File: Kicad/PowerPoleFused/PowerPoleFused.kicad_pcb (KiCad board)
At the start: 2 copper layers, 96.5 x 43.2 mm, 12 parts, among them J1 Anderson powerpole, J2 Anderson powerpole, J3 Anderson powerpole, J4 Anderson powerpole, J5 Anderson powerpole, J6 Anderson powerpole

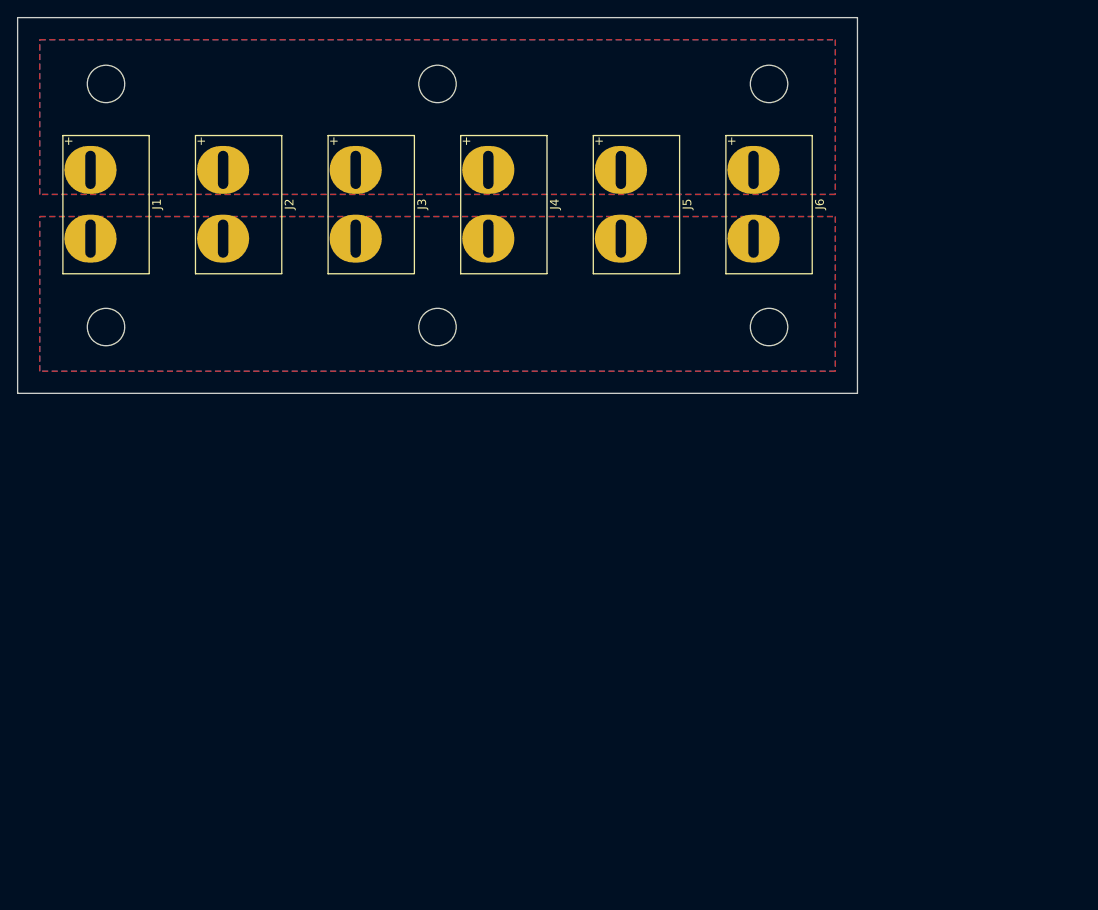
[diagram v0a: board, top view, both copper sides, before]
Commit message: Laid out board 1st attempt
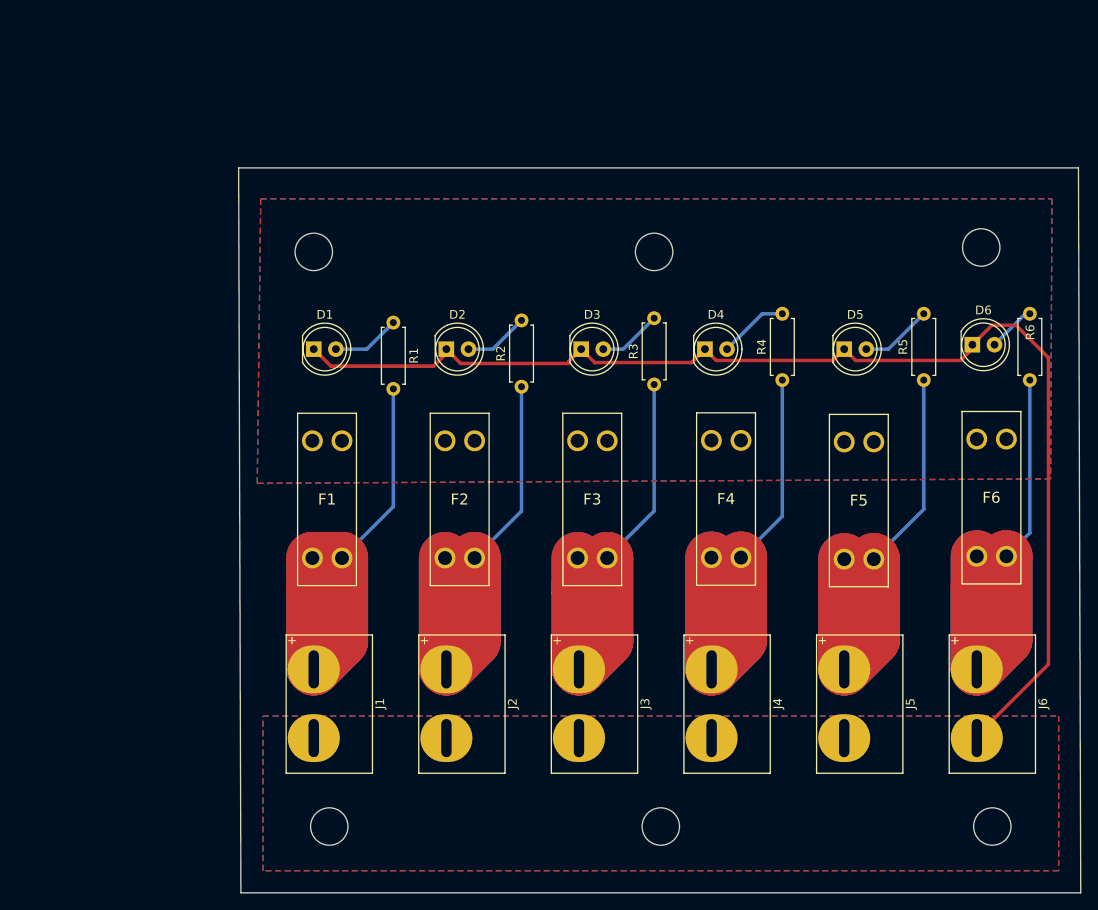
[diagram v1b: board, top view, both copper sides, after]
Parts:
- added D1: LED, LED_THT:LED_D5.0mm, F.Cu at (54.4, 50.8)
- added D2: LED, LED_THT:LED_D5.0mm, F.Cu at (69.6, 50.8)
- added D3: LED, LED_THT:LED_D5.0mm, F.Cu at (85.1, 50.8)
- added D4: LED, LED_THT:LED_D5.0mm, F.Cu at (99.3, 50.8)
- added D5: LED, LED_THT:LED_D5.0mm, F.Cu at (115.3, 50.8)
- added D6: LED, LED_THT:LED_D5.0mm, F.Cu at (130.0, 50.3)
- added F1: SamacSys_Parts_3557-20, Fuses:355720, F.Cu at (54.2, 74.8)
- added F2: SamacSys_Parts_3557-20, Fuses:355720, F.Cu at (69.4, 74.8)
- added F3: SamacSys_Parts_3557-20, Fuses:355720, F.Cu at (84.7, 74.8)
- added F4: SamacSys_Parts_3557-20, Fuses:355720, F.Cu at (100.1, 74.8)
- added F5: SamacSys_Parts_3557-20, Fuses:355720, F.Cu at (115.3, 74.9)
- added F6: SamacSys_Parts_3557-20, Fuses:355720, F.Cu at (130.6, 74.6)
- added R1: 2K2, Resistor_THT:R_Axial_DIN0207_L6.3mm_D2.5mm_P7.62mm_Horizontal, F.Cu at (63.5, 47.8)
- added R2: 2K2, Resistor_THT:R_Axial_DIN0207_L6.3mm_D2.5mm_P7.62mm_Horizontal, F.Cu at (78.2, 55.1)
- added R3: 2K2, Resistor_THT:R_Axial_DIN0207_L6.3mm_D2.5mm_P7.62mm_Horizontal, F.Cu at (93.5, 54.9)
- added R4: 2K2, Resistor_THT:R_Axial_DIN0207_L6.3mm_D2.5mm_P7.62mm_Horizontal, F.Cu at (108.2, 54.4)
- added R5: 2K2, Resistor_THT:R_Axial_DIN0207_L6.3mm_D2.5mm_P7.62mm_Horizontal, F.Cu at (124.5, 54.4)
- added R6: 2K2, Resistor_THT:R_Axial_DIN0207_L6.3mm_D2.5mm_P7.62mm_Horizontal, F.Cu at (136.7, 54.4)
- moved REF** 62.9 mm to (56.1, 105.7)
- moved REF** 62.9 mm to (94.2, 105.7)
- moved J1 62.9 mm to (54.4, 87.6)
- moved J2 62.9 mm to (69.6, 87.6)
- moved J3 62.9 mm to (84.8, 87.6)
- moved J4 62.9 mm to (100.1, 87.6)
- moved J5 62.9 mm to (115.3, 87.6)
- moved J6 62.9 mm to (130.6, 87.6)
- moved REF** 62.9 mm to (132.3, 105.7)
- moved REF** 31.5 mm to (93.5, 39.6)
- moved REF** 30.8 mm to (131.1, 39.1)
- moved REF** 30.7 mm to (54.4, 39.6)
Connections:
- net Net-(J1--ve) renamed 0
- J2 pad 1: Net-(J1-+ve) -> Net-(J2-+ve)
- J3 pad 1: Net-(J1-+ve) -> Net-(J3-+ve)
- J4 pad 1: Net-(J1-+ve) -> Net-(J4-+ve)
- J5 pad 1: Net-(J1-+ve) -> Net-(J5-+ve)
- J6 pad 1: Net-(J1-+ve) -> Net-(J6-+ve)
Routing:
- net 0: track 0.00 -> 141.3 mm
- net Net-(J4-+ve): track 0.00 -> 90.8 mm
- net Net-(J6-+ve): track 0.00 -> 90.6 mm
- net Net-(J1-+ve): track 0.00 -> 87.3 mm
- net Net-(J3-+ve): track 0.00 -> 81.3 mm
- net Net-(J5-+ve): track 0.00 -> 81.2 mm
- net Net-(J2-+ve): track 0.00 -> 80.7 mm
- net Net-(D5-A): track 0.00 -> 8.29 mm
- net Net-(D4-A): track 0.00 -> 8.04 mm
- net Net-(D1-A): track 0.00 -> 7.87 mm
- net Net-(D2-A): track 0.00 -> 7.46 mm
- net Net-(D3-A): track 0.00 -> 7.32 mm
- net Net-(D6-A): track 0.00 -> 5.54 mm
- added copper zone on B.Cu, net +12V
- added copper zone on F.Cu, net +12V
- removed copper zone on B.Cu, net Net-(J1-+ve)
- removed copper zone on F.Cu, net Net-(J1-+ve)
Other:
- board size 96.5 x 43.2 mm -> 96.8 x 83.3 mm
